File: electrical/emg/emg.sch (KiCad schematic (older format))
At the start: 75 parts, among them J1 USB_B, J10 Ref, J2 swd, J3 T3, J4 T3, J5 T3, J6 T3, J7 T3, J8 T3, J9 T3, P1 ~rst~, P2 bootldr, U1 stm32f405rgt6, U2 crystal-4pin, U3 my-NCP1117ST50T3G, U4 my-NCP1117ST50T3G, U5 TSV734IPT, U6 TSV734IPT

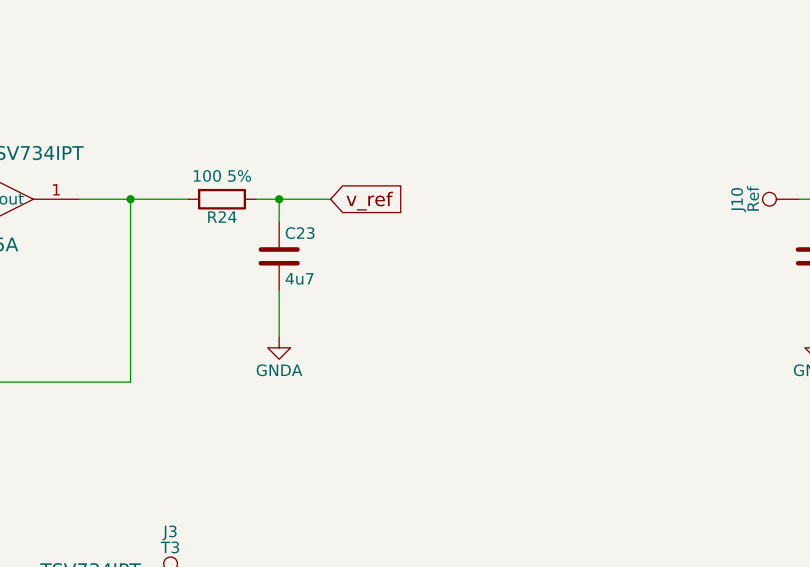
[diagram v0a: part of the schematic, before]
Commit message: a
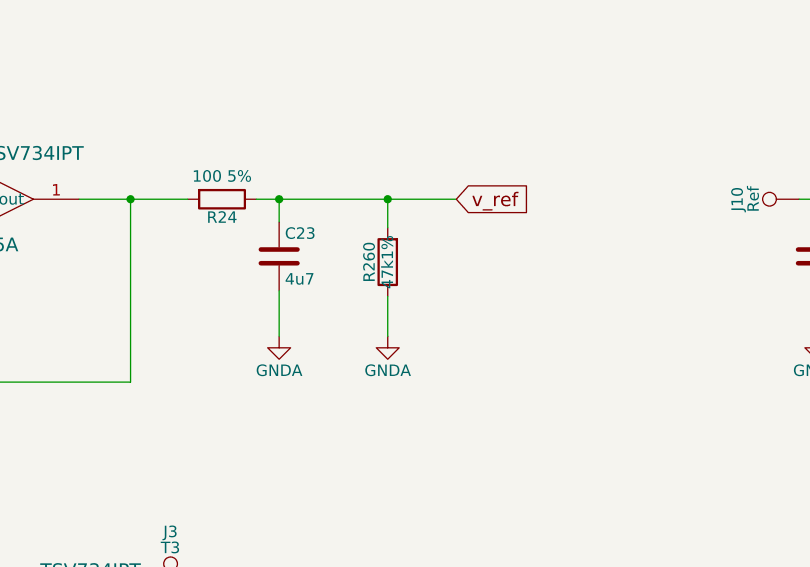
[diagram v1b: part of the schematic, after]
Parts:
- added R260: 47k1%, Resistor_SMD:R_0603_1608Metric, symbol R
- TP100, TP101, TP102, TP103: footprint (none) -> MountingHole:MountingHole_3.2mm_M3_DIN965_Pad
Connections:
- wire segments 223 -> 225
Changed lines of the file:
@@
 	1    0    0    -1
 $EndComp
-Text GLabel 19450 2250 2    60   Input ~ 0
+Text GLabel 20000 2250 2    60   Input ~ 0
 v_ref
 $Comp
@@
 $EndComp
 Wire Wire Line
-	19125 2250 19450 2250
+	19125 2250 20000 2250
 Wire Wire Line
 	19225 2350 19225 2250
@@
 F 0 "TP100" H 10000 9800 50  0000 C BNN
 F 1 "M3" H 10000 9750 50  0000 C CNN
-F 2 "" H 10000 9500 50  0001 C CNN
+F 2 "MountingHole:MountingHole_3.2mm_M3_DIN965_Pad" H 10000 9500 50  0001 C CNN
 F 3 "" H 10000 9500 50  0001 C CNN
 	1    10000 9500
@@
 $EndComp
 $Comp
-L GND #PWR?
+L GND #PWR048
 U 1 1 5BA50B5E
 P 10000 9700
-F 0 "#PWR?" H 10000 9450 50  0001 C CNN
+F 0 "#PWR048" H 10000 9450 50  0001 C CNN
 F 1 "GND" H 10000 9550 50  0000 C CNN
 F 2 "" H 10000 9700 60  0000 C CNN
@@
 F 0 "TP101" H 10200 9800 50  0000 C BNN
 F 1 "M3" H 10200 9750 50  0000 C CNN
-F 2 "" H 10200 9500 50  0001 C CNN
+F 2 "MountingHole:MountingHole_3.2mm_M3_DIN965_Pad" H 10200 9500 50  0001 C CNN
 F 3 "" H 10200 9500 50  0001 C CNN
 	1    10200 9500
@@
 $EndComp
 $Comp
-L GND #PWR?
+L GND #PWR049
 U 1 1 5BA514E3
 P 10200 9700
-F 0 "#PWR?" H 10200 9450 50  0001 C CNN
+F 0 "#PWR049" H 10200 9450 50  0001 C CNN
 F 1 "GND" H 10200 9550 50  0000 C CNN
 F 2 "" H 10200 9700 60  0000 C CNN
@@
 F 0 "TP102" H 10400 9800 50  0000 C BNN
 F 1 "M3" H 10400 9750 50  0000 C CNN
-F 2 "" H 10400 9500 50  0001 C CNN
+F 2 "MountingHole:MountingHole_3.2mm_M3_DIN965_Pad" H 10400 9500 50  0001 C CNN
 F 3 "" H 10400 9500 50  0001 C CNN
 	1    10400 9500
@@
 $EndComp
 $Comp
-L GND #PWR?
+L GND #PWR050
 U 1 1 5BA516D0
 P 10400 9700
-F 0 "#PWR?" H 10400 9450 50  0001 C CNN
+F 0 "#PWR050" H 10400 9450 50  0001 C CNN
 F 1 "GND" H 10400 9550 50  0000 C CNN
 F 2 "" H 10400 9700 60  0000 C CNN
@@
 F 0 "TP103" H 10600 9800 50  0000 C BNN
 F 1 "M3" H 10600 9750 50  0000 C CNN
-F 2 "" H 10600 9500 50  0001 C CNN
+F 2 "MountingHole:MountingHole_3.2mm_M3_DIN965_Pad" H 10600 9500 50  0001 C CNN
 F 3 "" H 10600 9500 50  0001 C CNN
 	1    10600 9500
@@
 $EndComp
 $Comp
-L GND #PWR?
+L GND #PWR051
 U 1 1 5BA516DD
 P 10600 9700
-F 0 "#PWR?" H 10600 9450 50  0001 C CNN
+F 0 "#PWR051" H 10600 9450 50  0001 C CNN
 F 1 "GND" H 10600 9550 50  0000 C CNN
 F 2 "" H 10600 9700 60  0000 C CNN
@@
 Wire Wire Line
 	10600 9500 10600 9700
+$Comp
+L R R260
+U 1 1 5B9E3524
+P 19700 2525
+F 0 "R260" V 19780 2525 50  0000 C CNN
+F 1 "47k1%" V 19700 2525 50  0000 C CNN
+F 2 "Resistor_SMD:R_0603_1608Metric" V 19630 2525 30  0001 C CNN
+F 3 "" H 19700 2525 30  0000 C CNN
+	1    19700 2525
+	-1   0    0    1
+$EndComp
+Wire Wire Line
+	19700 2250 19700 2375
+Connection ~ 19700 2250
+Wire Wire Line
+	19700 2675 19700 2850
+$Comp
+L GNDA #PWR052
+U 1 1 5B9E3E05
+P 19700 2850
+F 0 "#PWR052" H 19700 2600 50  0001 C CNN
+F 1 "GNDA" H 19700 2700 50  0000 C CNN
+F 2 "" H 19700 2850 50  0001 C CNN
+F 3 "" H 19700 2850 50  0001 C CNN
+	1    19700 2850
+	1    0    0    -1
+$EndComp
 $EndSCHEMATC

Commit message: Making two separate boards. One for ADC and the other one for preamplification.
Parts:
- removed J4, J5, J6, J9: T3, TestPoint:TestPoint_Pad_D1.0mm, symbol TEST_1P
- added J11, J12, J13, J4, J5, J6, J9: Conn_01x05, Pin_Headers:Pin_Header_Straight_1x05_Pitch1.27mm, symbol Conn_01x05
- added J14, J15, J16, J17: T3, TestPoint:TestPoint_Pad_D1.0mm, symbol TEST_1P
- C19: value 100n -> 2n2
- C24: value 2n2 -> 100n
- R17, R18, R19, R20, R21, R22, R23: value 10k 1% -> 1k 1%
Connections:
- net labels added: v_0, v_1, v_2, v_3, v_4, v_5, v_6
- wire segments 225 -> 280
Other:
- moved on the sheet: C25, J10, R25
